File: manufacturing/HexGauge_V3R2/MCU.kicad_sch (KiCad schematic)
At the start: 26 parts, among them SW2 SW_Panasonic_EVQPUC, SW2 SW_SPDT, U2 STM32F405RGT6, Y1 25MHz 12pF

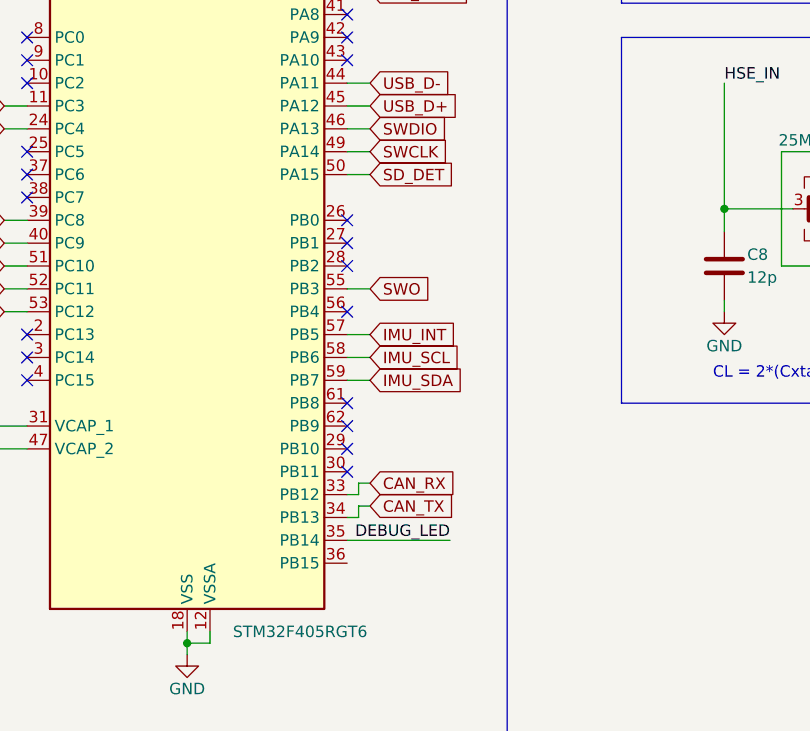
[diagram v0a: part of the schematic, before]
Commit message: upd board
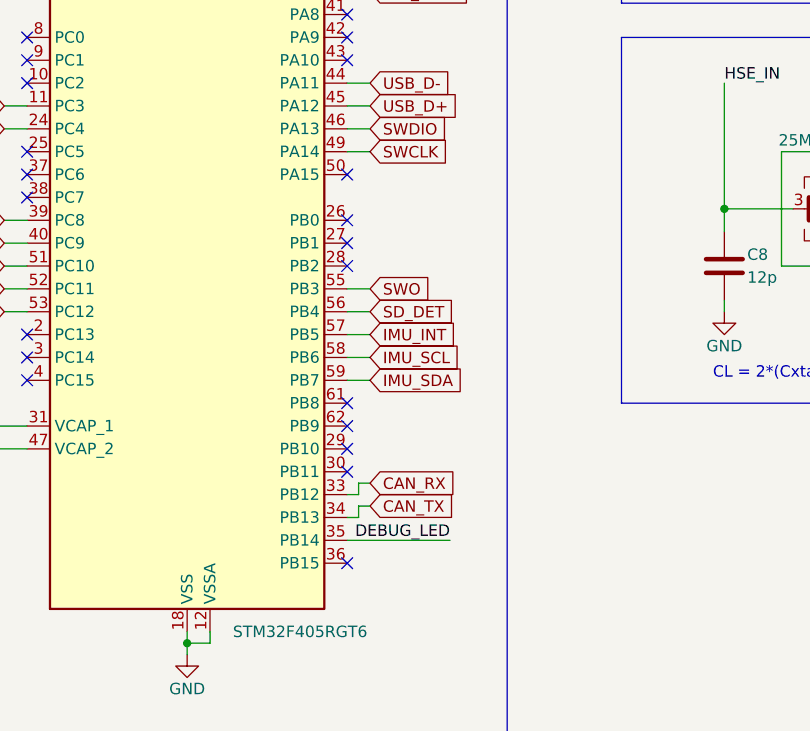
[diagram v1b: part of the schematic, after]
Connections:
- net SD_DET: now also U2.56 (PB4); no longer U2.50 (PA15)
- no-connect marks 23 -> 24
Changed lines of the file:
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@@
   (no_connect (at 121.92 138.43))
   (no_connect (at 121.92 118.11))
-  (no_connect (at 121.92 123.19))
+  (no_connect (at 121.92 107.95))
   (no_connect (at 121.92 140.97))
+  (no_connect (at 121.92 151.13))
   (no_connect (at 121.92 92.71))
   (no_connect (at 121.92 95.25))
@@
     (stroke (width 0) (type default))
   )
-  (wire (pts (xy 124.46 107.95) (xy 121.92 107.95))
-    (stroke (width 0) (type default))
-  )
   (wire (pts (xy 180.34 63.5) (xy 180.34 64.77))
     (stroke (width 0) (type default))
@@
   )
   (wire (pts (xy 123.19 146.05) (xy 121.92 146.05))
+    (stroke (width 0) (type default))
+  )
+  (wire (pts (xy 124.46 123.19) (xy 121.92 123.19))
     (stroke (width 0) (type default))
   )
@@
     )
   )
-  (global_label "SD_DET" (shape input) (at 124.46 107.95 0) (fields_autoplaced)
-    (effects (font (size 1.27 1.27)) (justify left))
-    (property "Intersheetrefs" "${INTERSHEET_REFS}" (at 134.1995 107.95 0)
-      (effects (font (size 1.27 1.27)) (justify left) hide)
-    )
+  (global_label "SD_DET" (shape input) (at 124.46 123.19 0) (fields_autoplaced)
+    (effects (font (size 1.27 1.27)) (justify left))
+    (property "Intersheetrefs" "${INTERSHEET_REFS}" (at 134.1995 123.19 0)
+      (effects (font (size 1.27 1.27)) (justify left) hide)
+    )

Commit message: upd fields
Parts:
- C1, C10, C2, C3, C4, C5, C6, C7, C8, C9, D1, R1, R? (x2), U2, Y1: Dist (none) -> LCSC
- SW2: Dist (none) -> Mouser
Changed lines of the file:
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@@
+      (effects (font (size 1.27 1.27)) hide)
+    )
+    (property "Dist" "LCSC" (at 39.37 154.94 0)
       (effects (font (size 1.27 1.27)) hide)
     )
@@
       (effects (font (size 1.27 1.27)) hide)
     )
+    (property "Dist" "LCSC" (at 45.72 54.61 0)
+      (effects (font (size 1.27 1.27)) hide)
+    )
     (pin "1")
     (pin "2")
@@
       (effects (font (size 1.27 1.27)) hide)
     )
+    (property "Dist" "Mouser" (at 220.98 66.04 0)
+      (effects (font (size 1.27 1.27)) hide)
+    )
     (pin "1")
     (pin "2")
@@
       (effects (font (size 1.27 1.27)) hide)
     )
+    (property "Dist" "LCSC" (at 76.2 143.51 0)
+      (effects (font (size 1.27 1.27)) hide)
+    )
     (pin "1")
     (pin "2")
@@
     )
     (property "LCSC Part #" "C1525" (at 57.15 54.61 0)
+      (effects (font (size 1.27 1.27)) hide)
+    )
+    (property "Dist" "LCSC" (at 57.15 54.61 0)
       (effects (font (size 1.27 1.27)) hide)
     )
@@
       (effects (font (size 1.27 1.27)) hide)
     )
+    (property "Dist" "Mouser" (at 162.56 63.5 0)
+      (effects (font (size 1.27 1.27)) hide)
+    )
     (pin "1")
     (pin "2")
@@
     )
     (property "LCSC Part #" "C15742" (at 104.14 113.03 0)
+      (effects (font (size 1.27 1.27)) hide)
+    )
+    (property "Dist" "LCSC" (at 104.14 113.03 0)
       (effects (font (size 1.27 1.27)) hide)
     )
@@
       (effects (font (size 1.27 1.27)) hide)
     )
+    (property "Dist" "LCSC" (at 78.74 54.61 0)
+      (effects (font (size 1.27 1.27)) hide)
+    )
     (pin "1")
     (pin "2")
@@
     )
     (property "LCSC Part #" "C25077" (at 173.99 63.5 0)
+      (effects (font (size 1.27 1.27)) hide)
+    )
+    (property "Dist" "LCSC" (at 173.99 63.5 0)
       (effects (font (size 1.27 1.27)) hide)
     )
@@
       (effects (font (size 1.27 1.27)) hide)
     )
+    (property "Dist" "LCSC" (at 175.26 111.76 0)
+      (effects (font (size 1.27 1.27)) hide)
+    )
     (pin "1")
     (pin "2")
@@
       (effects (font (size 1.27 1.27)) hide)
     )
+    (property "Dist" "LCSC" (at 66.04 143.51 0)
+      (effects (font (size 1.27 1.27)) hide)
+    )
     (pin "1")
     (pin "2")
@@
       (effects (font (size 1.27 1.27)) hide)
     )
+    (property "Dist" "LCSC" (at 118.11 54.61 0)
+      (effects (font (size 1.27 1.27)) hide)
+    )
     (pin "1")
     (pin "2")
@@
     )
     (property "LCSC Part #" "C23630" (at 180.34 68.58 0)
+      (effects (font (size 1.27 1.27)) hide)
+    )
+    (property "Dist" "LCSC" (at 180.34 68.58 0)
       (effects (font (size 1.27 1.27)) hide)
     )
@@
     )
     (property "LCSC Part #" "C25744" (at 180.34 54.61 0)
+      (effects (font (size 1.27 1.27)) hide)
+    )
+    (property "Dist" "LCSC" (at 180.34 54.61 0)
       (effects (font (size 1.27 1.27)) hide)
     )
@@
       (effects (font (size 1.27 1.27)) hide)
     )
+    (property "Dist" "LCSC" (at 223.52 115.57 0)
+      (effects (font (size 1.27 1.27)) hide)
+    )
     (pin "1")
     (pin "2")
@@
     )
     (property "LCSC Part #" "C25077" (at 220.98 54.61 0)
+      (effects (font (size 1.27 1.27)) hide)
+    )
+    (property "Dist" "LCSC" (at 220.98 54.61 0)
       (effects (font (size 1.27 1.27)) hide)
     )
@@
       (effects (font (size 1.27 1.27)) hide)
     )
+    (property "Dist" "" (at 194.31 63.5 0)
+      (effects (font (size 1.27 1.27)) hide)
+    )
     (pin "1")
     (pin "2")
@@
       (effects (font (size 1.27 1.27)) hide)
     )
+    (property "Dist" "LCSC" (at 45.72 154.94 0)
+      (effects (font (size 1.27 1.27)) hide)
+    )
     (pin "1")
     (pin "2")
@@
     )
     (property "LCSC Part #" "C1525" (at 67.31 54.61 0)
+      (effects (font (size 1.27 1.27)) hide)
+    )
+    (property "Dist" "LCSC" (at 67.31 54.61 0)
       (effects (font (size 1.27 1.27)) hide)
     )
@@
       (effects (font (size 1.27 1.27)) hide)
     )
+    (property "Dist" "LCSC" (at 88.9 54.61 0)
+      (effects (font (size 1.27 1.27)) hide)
+    )
     (pin "1")
     (pin "2")
@@
       (effects (font (size 1.27 1.27)) hide)
     )
+    (property "Dist" "LCSC" (at 223.52 106.68 0)
+      (effects (font (size 1.27 1.27)) hide)
+    )
     (pin "1")
     (pin "2")
@@
       (effects (font (size 1.27 1.27)) hide)
     )
+    (property "Dist" "LCSC" (at 34.29 54.61 0)
+      (effects (font (size 1.27 1.27)) hide)
+    )
     (pin "1")
     (pin "2")
@@
     )
     (property "LCSC Part #" "C1547" (at 163.83 118.11 0)
+      (effects (font (size 1.27 1.27)) hide)
+    )
+    (property "Dist" "LCSC" (at 163.83 118.11 0)
       (effects (font (size 1.27 1.27)) hide)
     )
@@
       (effects (font (size 1.27 1.27)) hide)
     )
+    (property "Dist" "LCSC" (at 162.56 72.39 0)
+      (effects (font (size 1.27 1.27)) hide)
+    )
     (pin "1")
     (pin "2")
@@
       (effects (font (size 1.27 1.27)) hide)
     )
+    (property "Dist" "LCSC" (at 184.15 105.41 0)
+      (effects (font (size 1.27 1.27)) hide)
+    )
     (pin "1")
     (pin "2")
@@
       (effects (font (size 1.27 1.27)) hide)
     )
+    (property "Dist" "LCSC" (at 184.15 118.11 0)
+      (effects (font (size 1.27 1.27)) hide)
+    )
